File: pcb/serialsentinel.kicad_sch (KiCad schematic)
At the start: 49 parts, among them J2 Bus_PCI_Express_x1, J3 REL1, J4 REL1, J5 REL2, J6 REL2, K2 G6K-2F-Y DC3, K3 G6K-2F-Y DC3, Q2 MMBT3904, Q3 MMBT3904, Q4 MMBT3904, Q5 MMBT3904, SW1 RESET, U1 CH382L, U2 XC6206P182MR, U3 ESP32-C3-WROOM-02U

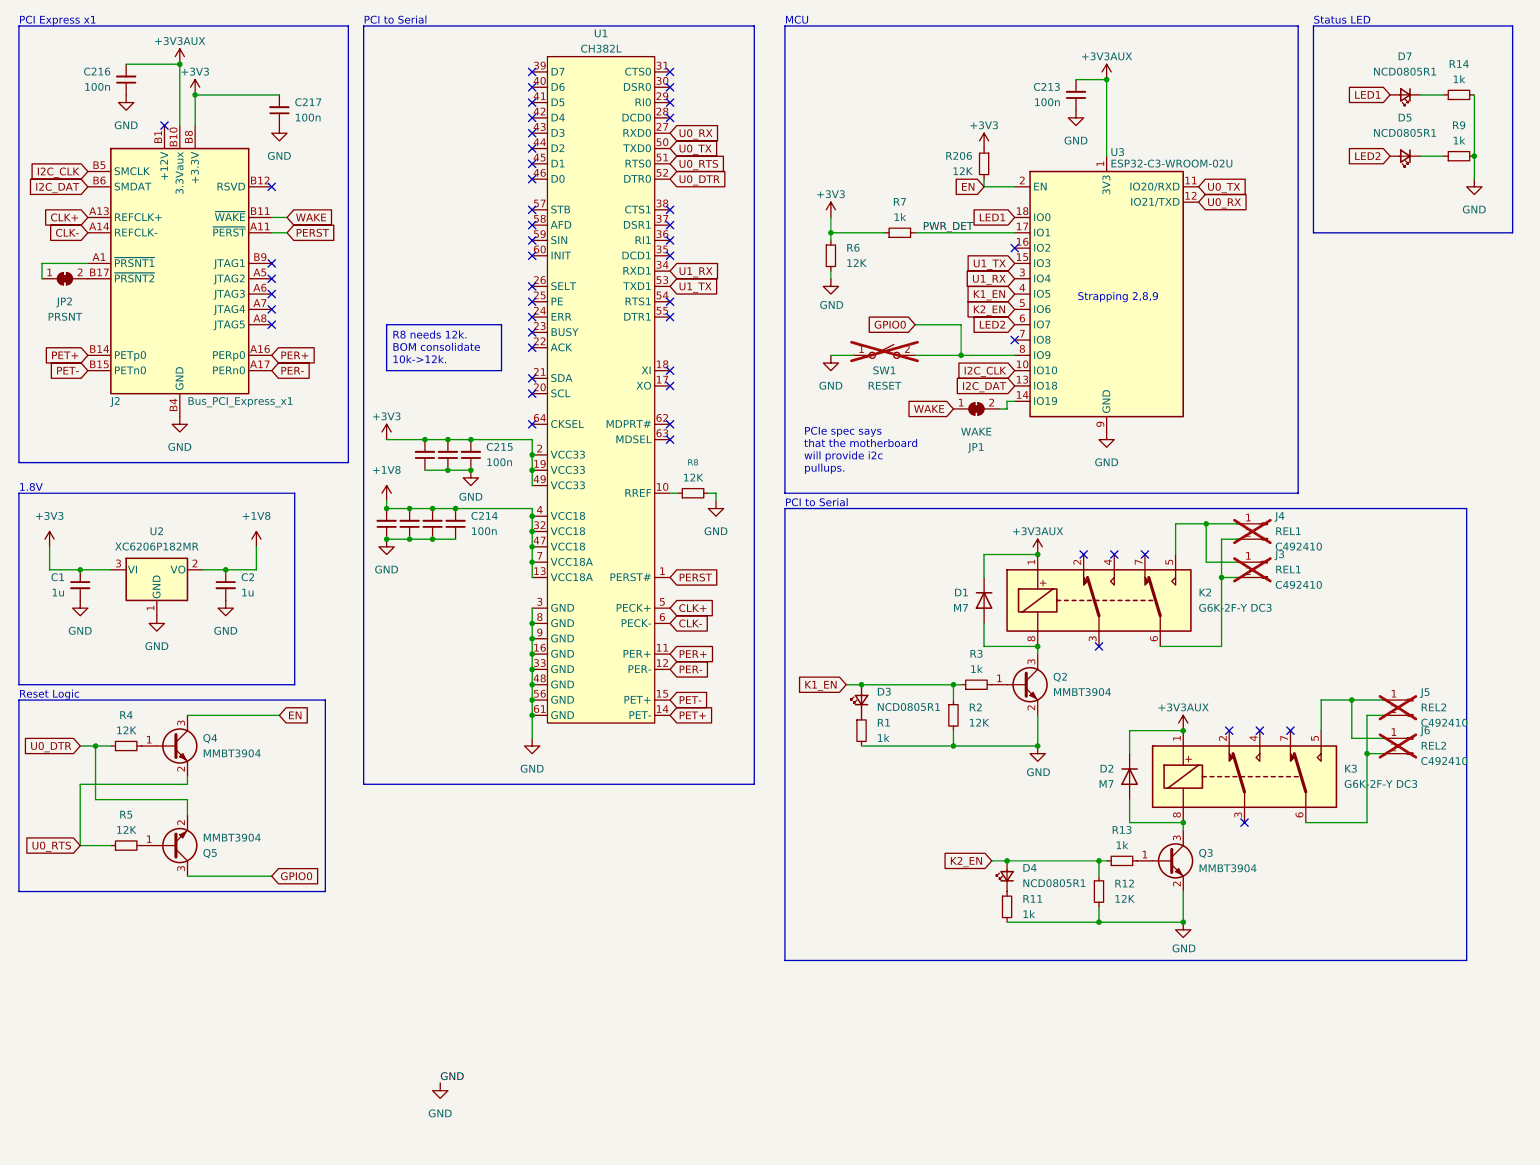
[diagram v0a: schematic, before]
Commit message: fixes
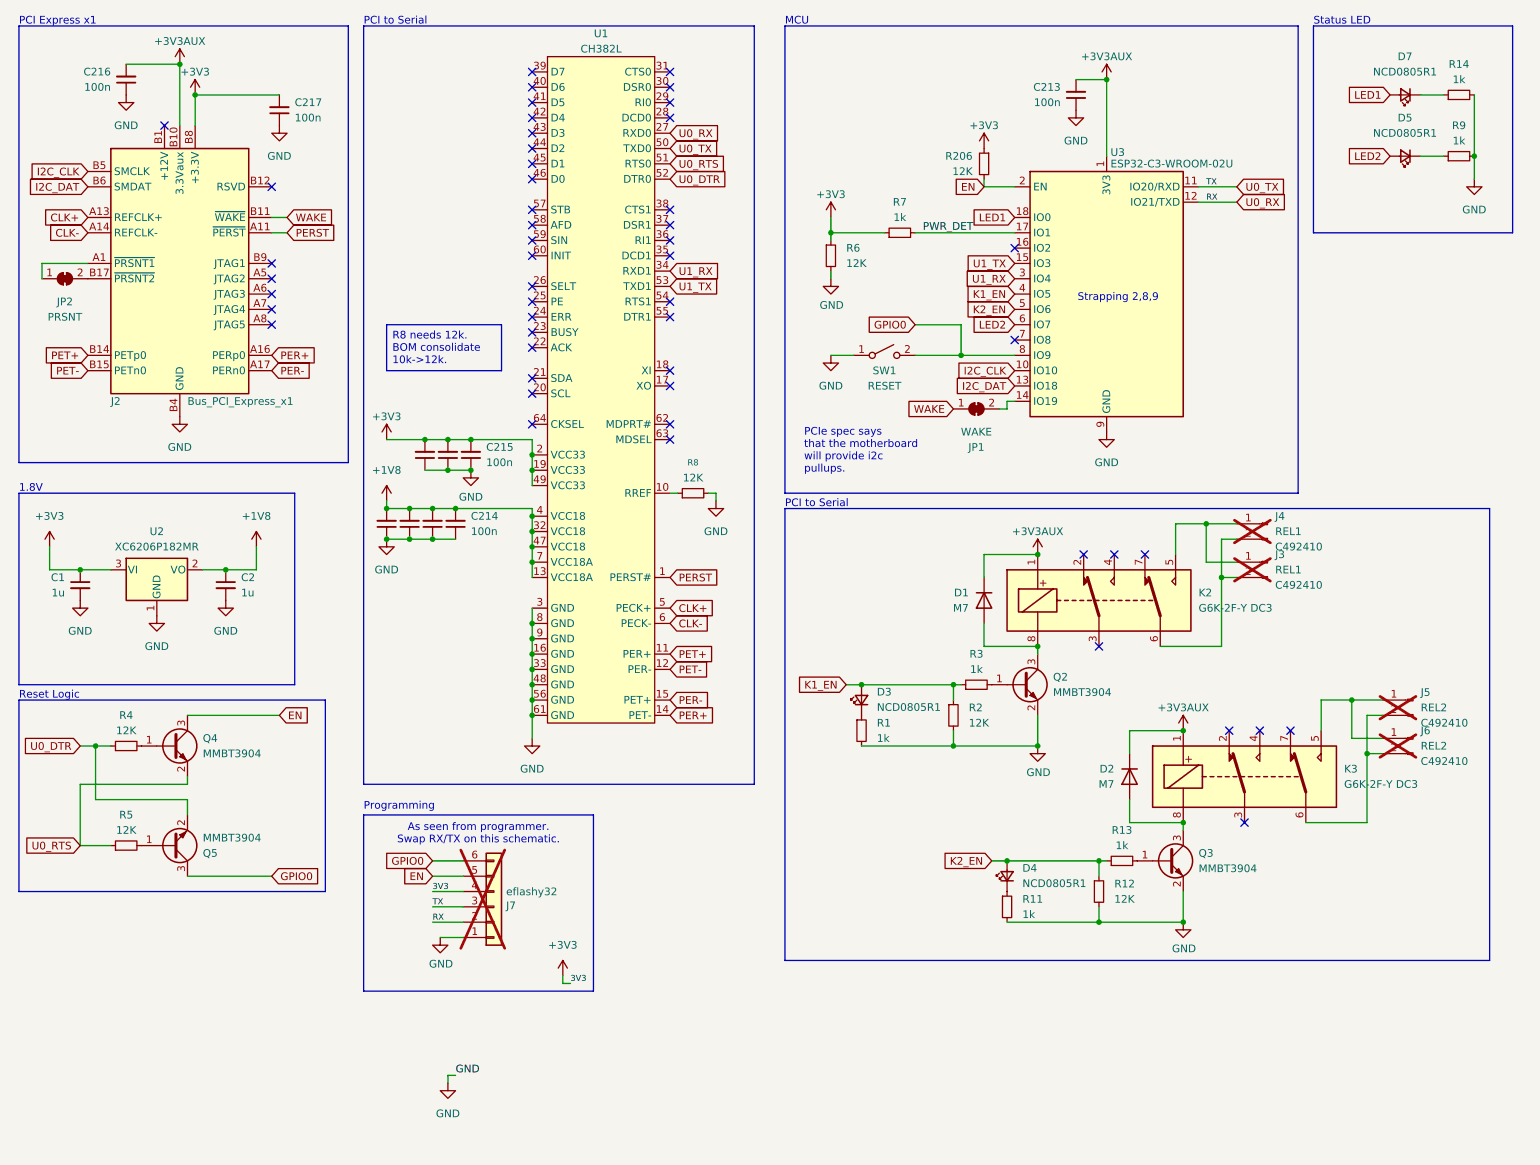
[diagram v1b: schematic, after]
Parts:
- added J7: eflashy32, Connector_PinHeader_2.54mm:PinHeader_1x06_P2.54mm_Vertical, symbol Connector_Generic:Conn_01x06
- SW1: now fitted
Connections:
- net +3V3: now also J7.4 (Pin_4)
- net EN: now also J7.5 (Pin_5)
- net GND: now also J7.1 (Pin_1)
- net GPIO0: now also J7.6 (Pin_6)
- net PER+: now also U1.14 (PET-); no longer U1.11 (PER+)
- net PER-: now also U1.15 (PET+); no longer U1.12 (PER-)
- net PET+: now also U1.11 (PER+); no longer U1.14 (PET-)
- net PET-: now also U1.12 (PER-); no longer U1.15 (PET+)
- net U0_RX: now also J7.2 (Pin_2)
- net U0_TX: now also J7.3 (Pin_3)
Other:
- note added: "As seen from programmer. Swap RX/TX on this schematic."
- note added: "Programming"

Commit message: towards v3!
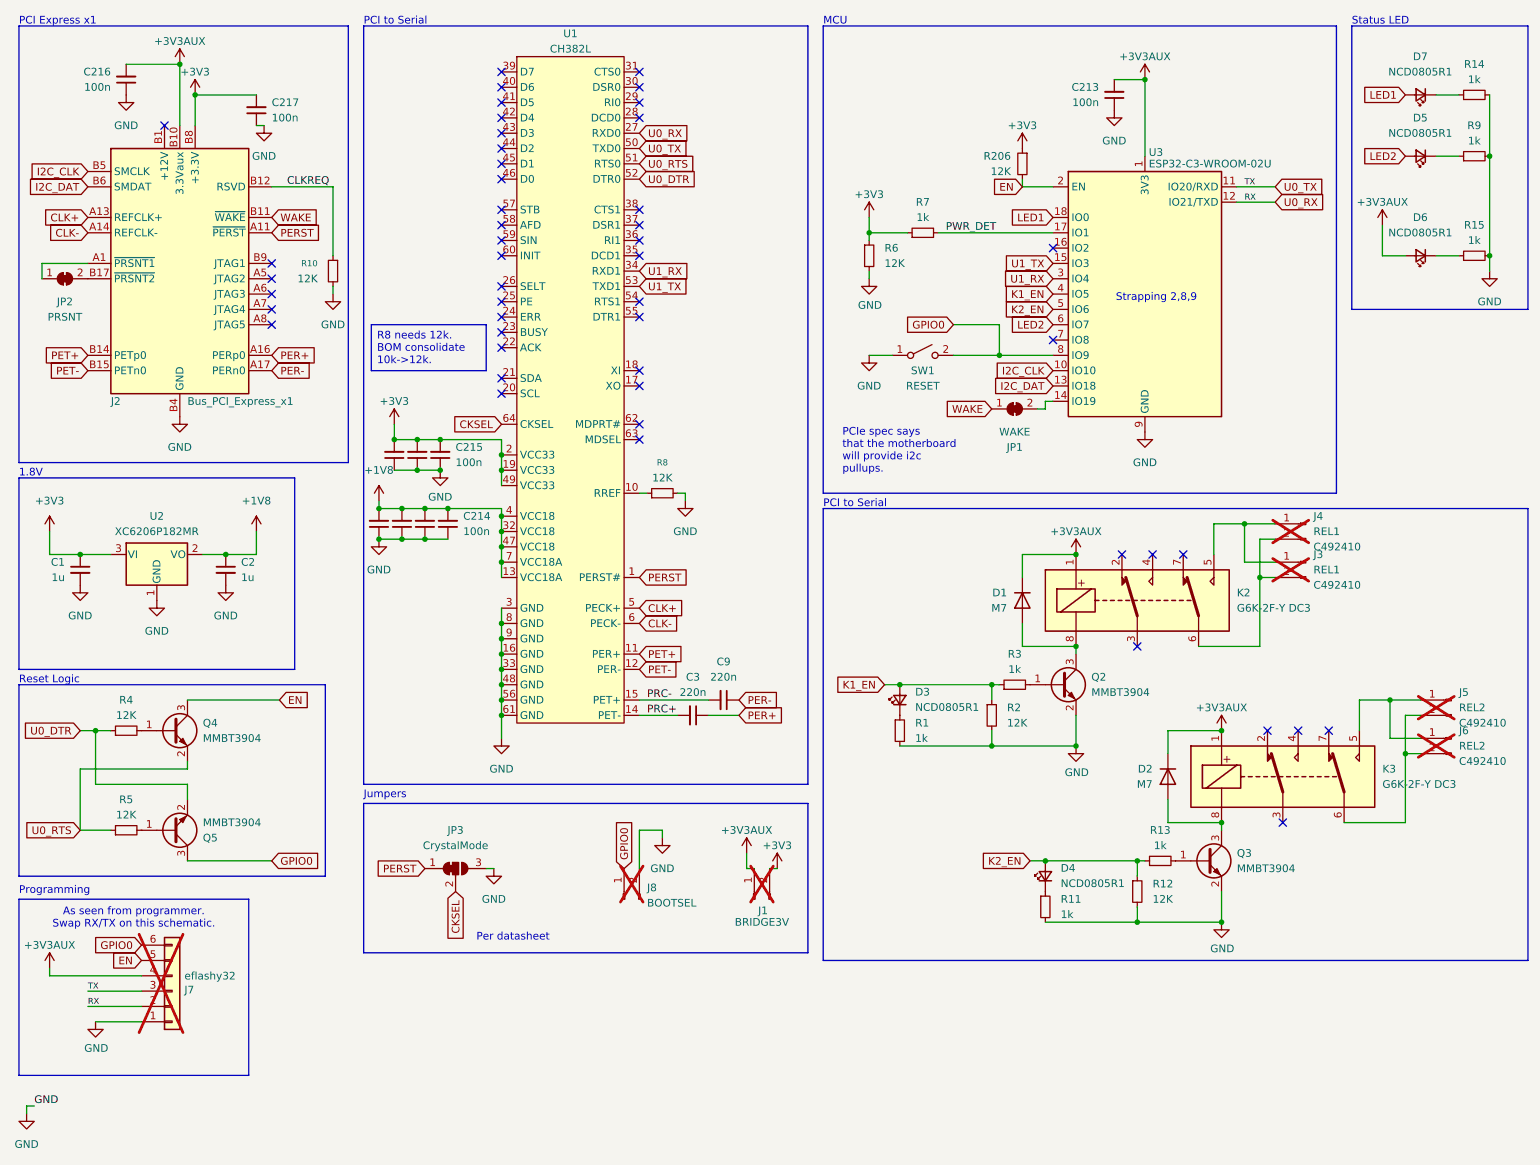
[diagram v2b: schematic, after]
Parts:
- added C3, C9: 220n, Capacitor_SMD:C_0402_1005Metric, symbol Device:C_Small
- added D6: NCD0805R1, LED_SMD:LED_0805_2012Metric, symbol Device:LED_Small
- added J1: BRIDGE3V, Connector_PinHeader_2.54mm:PinHeader_1x02_P2.54mm_Vertical, symbol Connector:Conn_01x02_Pin
- added J8: BOOTSEL, Connector_PinHeader_2.54mm:PinHeader_1x02_P2.54mm_Vertical, symbol Connector:Conn_01x02_Pin
- added JP3: CrystalMode, Jumper:SolderJumper-3_P1.3mm_Bridged12_RoundedPad1.0x1.5mm, symbol Jumper:SolderJumper_3_Bridged12
- added R10: 12K, Resistor_SMD:R_0402_1005Metric, symbol Device:R_Small
- added R15: 1k, Resistor_SMD:R_0402_1005Metric, symbol Device:R_Small
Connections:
- net +3V3: now also J1.2 (Pin_2); no longer J7.4 (Pin_4)
- net +3V3AUX: now also J7.4 (Pin_4), D6.2 (A), J1.1 (Pin_1)
- net GND: now also J8.2 (Pin_2), JP3.3 (B), R10.2, R15.2
- net GPIO0: now also J8.1 (Pin_1)
- net PER+: now also C3.1; no longer U1.14 (PET-)
- net PER-: now also C9.1; no longer U1.15 (PET+)
- net PERST: now also JP3.1 (A)
- net CKSEL: now reaches U1.64 (CKSEL)
- net CKSEL: now also JP3.2 (C)
- net CLKREQ: now reaches J2.B12 (RSVD)
- net CLKREQ: now also R10.1
- new net: D6.1 (K), R15.1
- new net PRC+: C3.2, U1.14 (PET-)
- new net PRC-: C9.2, U1.15 (PET+)
- no-connect marks 51 -> 49
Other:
- note added: "Jumpers"
- note added: "Per datasheet"
- moved on the sheet: C1, C2, C213, C214, C215, C217, D1, D2, D3, D4, D5, D7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
